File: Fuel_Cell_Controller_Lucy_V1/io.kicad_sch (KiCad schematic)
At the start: 52 parts, among them J3 DE9_Receptacle, J4 DA15_Receptacle_MountingHoles, J6 Screw_Terminal_01x02, J7 USB_B_Micro, U14 FT234XD-R, U17 AD8603, U6 USBLC6-2SC6, U7 MCP1501-33E/SN, U8 AD8603, U9 AD8603, U9 MCP2542FD-E/SN

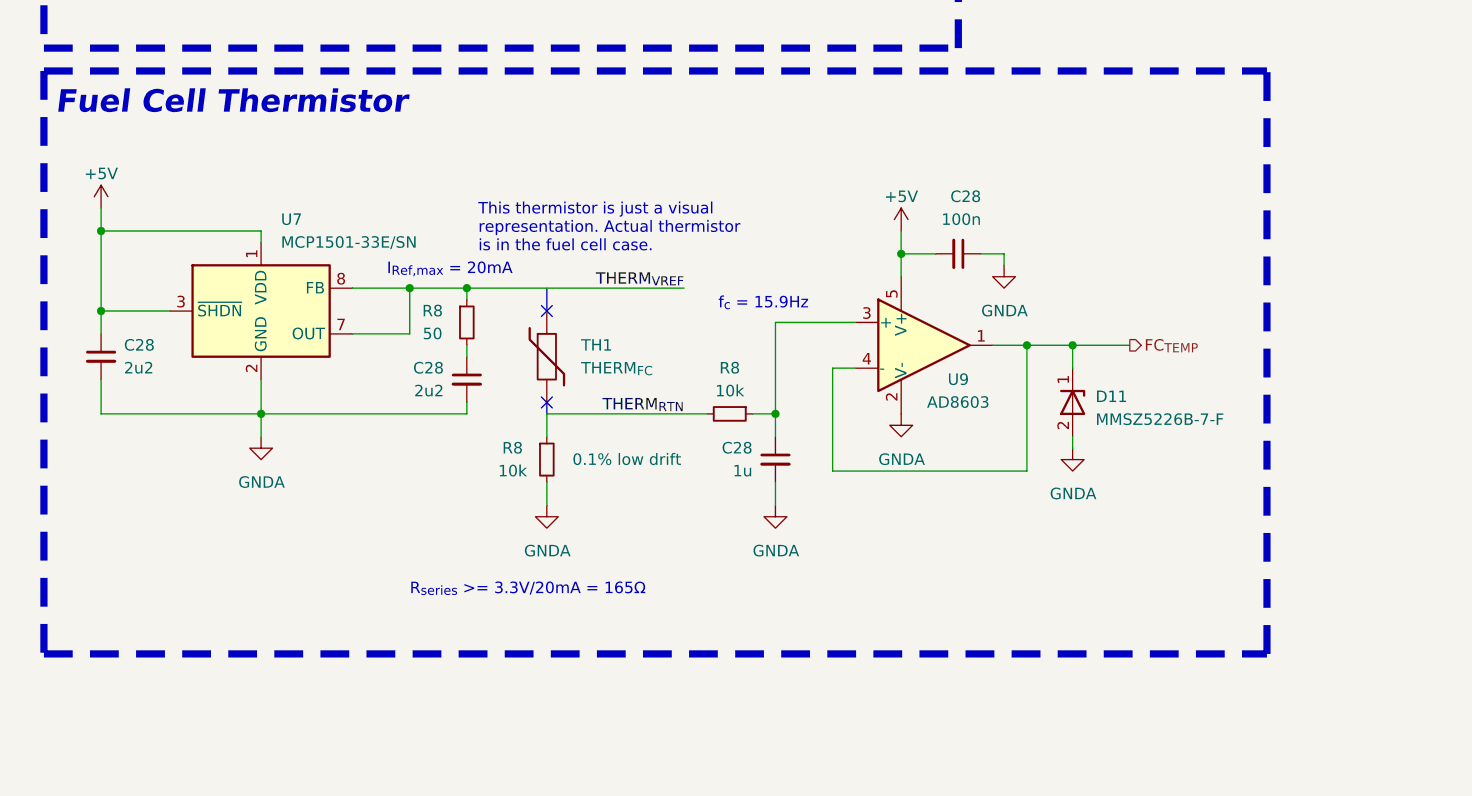
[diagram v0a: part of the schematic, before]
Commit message: things
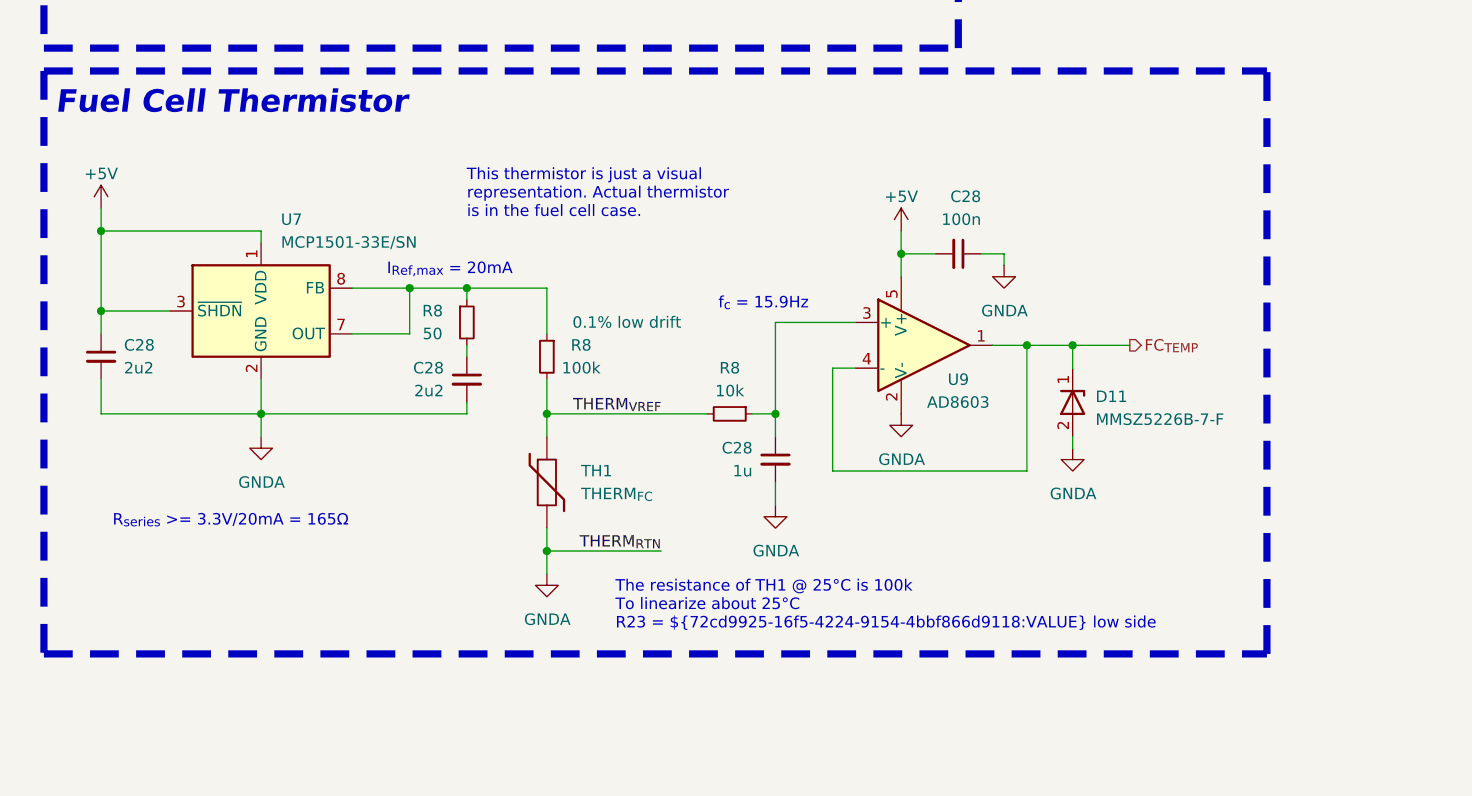
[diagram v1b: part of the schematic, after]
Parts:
- R8: value 10k -> 100k
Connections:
- net GNDA: now also J4.13 (P13), TH1.2; no longer R8.2
- net THERM_{VREF}: now also R8.2, R8.2, TH1.1; no longer R8.1, U7.7 (OUT), U7.8 (FB)
- removed net THERM_{RTN}: J4.13 (P13), R8.1, R8.2
- new net: R8.1, R8.1, U7.7 (OUT), U7.8 (FB)
- no-connect marks 9 -> 7
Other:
- note added: "The resistance of TH1 @ 25°C is 100k To linearize about 25°C R23 = ${72cd9925-16f5-4224-9154-4bbf866d9118:VALUE} low side"
- moved on the sheet: R8, TH1
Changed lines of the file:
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@@
   (junction (at 246.38 63.5) (diameter 0) (color 0 0 0 0)
   )
+  (junction (at 69.85 156.21) (diameter 0) (color 0 0 0 0)
+  )
   (junction (at 228.6 54.61) (diameter 0) (color 0 0 0 0)
   )
@@
   (junction (at 297.18 210.82) (diameter 0) (color 0 0 0 0)
   )
+  (junction (at 69.85 171.45) (diameter 0) (color 0 0 0 0)
+  )
   (junction (at 302.26 31.75) (diameter 0) (color 0 0 0 0)
   )
@@
   )
   (no_connect (at 353.06 53.34))
-  (no_connect (at 69.85 154.94))
   (no_connect (at 330.2 43.18))
-  (no_connect (at 69.85 144.78))
   (no_connect (at 389.89 205.74))
   (no_connect (at 330.2 35.56))
@@
     (stroke (width 0) (type default))
   )
-  (wire (pts (xy 60.96 142.24) (xy 85.09 142.24))
+  (wire (pts (xy 60.96 142.24) (xy 69.85 142.24))
     (stroke (width 0) (type default))
   )
@@
     (stroke (width 0) (type default))
   )
-  (polyline (pts (xy 69.85 142.24) (xy 69.85 144.78))
-    (stroke (width 0) (type default))
-  )
   (wire (pts (xy 328.93 114.3) (xy 356.87 114.3))
     (stroke (width 0) (type default))
@@
     (stroke (width 0) (type default))
   )
+  (wire (pts (xy 69.85 142.24) (xy 69.85 147.32))
+    (stroke (width 0) (type default))
+  )
   (wire (pts (xy 311.15 200.66) (xy 313.69 200.66))
     (stroke (width 0) (type default))
@@
     (stroke (width 0) (type default))
   )
+  (wire (pts (xy 69.85 152.4) (xy 69.85 156.21))
+    (stroke (width 0) (type default))
+  )
   (wire (pts (xy 389.89 203.2) (xy 387.35 203.2))
     (stroke (width 0) (type default))
@@
     (stroke (width 0.8) (type dash))
   )
-  (polyline (pts (xy 69.85 154.94) (xy 69.85 156.21))
-    (stroke (width 0) (type default))
-  )
   (wire (pts (xy 68.58 80.01) (xy 68.58 81.28))
     (stroke (width 0) (type default))
@@
     (stroke (width 0.8) (type dash))
   )
-  (wire (pts (xy 69.85 163.83) (xy 69.85 166.37))
+  (wire (pts (xy 69.85 171.45) (xy 69.85 173.99))
     (stroke (width 0) (type default))
   )
@@
     (stroke (width 0) (type default))
   )
+  (wire (pts (xy 69.85 171.45) (xy 82.55 171.45))
+    (stroke (width 0) (type default))
+  )
   (polyline (pts (xy 13.97 67.31) (xy 87.63 67.31))
     (stroke (width 0.8) (type dash))
@@
     (stroke (width 0) (type default))
   )
+  (wire (pts (xy 69.85 168.91) (xy 69.85 171.45))
+    (stroke (width 0) (type default))
+  )
   (wire (pts (xy 314.96 59.69) (xy 314.96 62.23))
     (stroke (width 0) (type default))
@@
   )
   (text "This thermistor is just a visual\nrepresentation. Actual thermistor\nis in the fuel cell case."
-    (at 62.23 138.43 0)
+    (at 60.96 134.62 0)
     (effects (font (size 1.27 1.27)) (justify left bottom))
   )
@@
     (effects (font (size 1.27 1.27)) (justify left bottom))
   )
+  (text "The resistance of TH1 @ 25°C is 100k\nTo linearize about 25°C\nR23 = ${72cd9925-16f5-4224-9154-4bbf866d9118:VALUE} low side"
+    (at 77.47 180.34 0)
+    (effects (font (size 1.27 1.27)) (justify left bottom))
+  )
   (text "FTDI - TTL to USB" (at 245.11 163.83 0)
     (effects (font (size 2.5 2.5) (thickness 0.5) bold italic) (justify left bottom))
@@
     (effects (font (size 1.27 1.27)) (justify left bottom))
   )
-  (text "R_{series} >= 3.3V/20mA = 165Ω" (at 54.61 176.53 0)
+  (text "R_{series} >= 3.3V/20mA = 165Ω" (at 21.59 168.91 0)
     (effects (font (size 1.27 1.27)) (justify left bottom))
   )
@@
     (effects (font (size 1.27 1.27)) (justify left bottom))
   )
-  (label "THERM_{RTN}" (at 85.09 156.21 180) (fields_autoplaced)
+  (label "THERM_{RTN}" (at 82.55 171.45 180) (fields_autoplaced)
     (effects (font (size 1.27 1.27)) (justify right bottom))
   )
@@
     (effects (font (size 1.27 1.27)) (justify right bottom))
   )
-  (label "THERM_{VREF}" (at 85.09 142.24 180) (fields_autoplaced)
+  (label "THERM_{VREF}" (at 82.55 156.21 180) (fields_autoplaced)
     (effects (font (size 1.27 1.27)) (justify right bottom))
   )
@@
     )
   )
-  (symbol (lib_id "Device:R_Small") (at 69.85 161.29 0) (unit 1)
+  (symbol (lib_id "Device:R_Small") (at 69.85 149.86 0) (mirror y) (unit 1)
     (in_bom yes) (on_board yes) (dnp no)
-    (property "Reference" "R8" (at 66.04 160.02 0)
+    (property "Reference" "R8" (at 73.66 148.59 0)
       (effects (font (size 1.27 1.27)))
     )
-    (property "Value" "10k" (at 66.04 162.56 0)
+    (property "Value" "100k" (at 73.66 151.13 0)
       (effects (font (size 1.27 1.27)))
     )
-    (property "Footprint" "Resistor_SMD:R_0603_1608Metric" (at 69.85 161.29 0)
+    (property "Footprint" "Resistor_SMD:R_0603_1608Metric" (at 69.85 149.86 0)
       (effects (font (size 1.27 1.27)) hide)
     )
-    (property "Datasheet" "~" (at 69.85 161.29 0)
+    (property "Datasheet" "~" (at 69.85 149.86 0)
       (effects (font (size 1.27 1.27)) hide)
     )
-    (property "Desc" "0.1% low drift" (at 78.74 161.29 0)
+    (property "Desc" "0.1% low drift" (at 78.74 146.05 0)
       (effects (font (size 1.27 1.27)))
     )
@@
     )
   )
-  (symbol (lib_id "power:GNDA") (at 69.85 166.37 0) (mirror y) (unit 1)
+  (symbol (lib_id "power:GNDA") (at 69.85 173.99 0) (mirror y) (unit 1)
     (in_bom yes) (on_board yes) (dnp no)
-    (property "Reference" "#PWR023" (at 69.85 172.72 0)
+    (property "Reference" "#PWR023" (at 69.85 180.34 0)
       (effects (font (size 1.27 1.27)) hide)
     )
-    (property "Value" "GNDA" (at 67.31 171.45 0)
+    (property "Value" "GNDA" (at 67.31 179.07 0)
       (effects (font (size 1.27 1.27)) (justify right))
     )
-    (property "Footprint" "" (at 69.85 166.37 0)
+    (property "Footprint" "" (at 69.85 173.99 0)
       (effects (font (size 1.27 1.27)) hide)
     )
-    (property "Datasheet" "" (at 69.85 166.37 0)
+    (property "Datasheet" "" (at 69.85 173.99 0)
       (effects (font (size 1.27 1.27)) hide)
     )
@@
     )
   )
-  (symbol (lib_id "Device:Thermistor") (at 69.85 149.86 0) (unit 1)
+  (symbol (lib_id "Device:Thermistor") (at 69.85 163.83 0) (unit 1)
     (in_bom no) (on_board no) (dnp no) (fields_autoplaced)
-    (property "Reference" "TH1" (at 73.66 148.59 0)
+    (property "Reference" "TH1" (at 73.66 162.56 0)
       (effects (font (size 1.27 1.27)) (justify left))
     )
-    (property "Value" "THERM_{FC}" (at 73.66 151.13 0)
+    (property "Value" "THERM_{FC}" (at 73.66 165.1 0)
       (effects (font (size 1.27 1.27)) (justify left))
     )
-    (property "Footprint" "" (at 69.85 149.86 0)
+    (property "Footprint" "" (at 69.85 163.83 0)
       (effects (font (size 1.27 1.27)) hide)
     )
-    (property "Datasheet" "~" (at 69.85 149.86 0)
+    (property "Datasheet" "~" (at 69.85 163.83 0)
       (effects (font (size 1.27 1.27)) hide)
     )
